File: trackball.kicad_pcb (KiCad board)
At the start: 4 copper layers, 65 x 85 mm, 255 parts, among them J2 ZX-PM2.0-2-4PY, Q1 XR2302, Q2 XR2302, Q4 XR2302, SW1 HX TC-5608-Y, SW2 HX TC-5608-Y, SW3 HX TC-5608-Y, SW4 HX TC-5608-Y, SW5 HX TC-5608-Y, SW6 HX TC-5608-Y, SW7 HX TC-5608-Y, SW8 HX TC-5608-Y, SW9 TS-1010-C-A, U1 USB-TYPE-C-017, U10 WS2812B, U11 WS2812B, U12 WS2812B, U13 WS2812B, U14 WS2812B, U15 WS2812B, U16 WS2812B, U17 WS2812B, U18 WS2812B, U19 WS2812B, U2 SY80004DQD, U20 WS2812B, U21 WS2812B, U3 SY80004DQD, U4 PMW3610, U5 PMW3610, U6 WS2812B, U7 WS2812B, U8 WS2812B, U9 WS2812B, X1 XL7EL89CKI-111YLC-32M

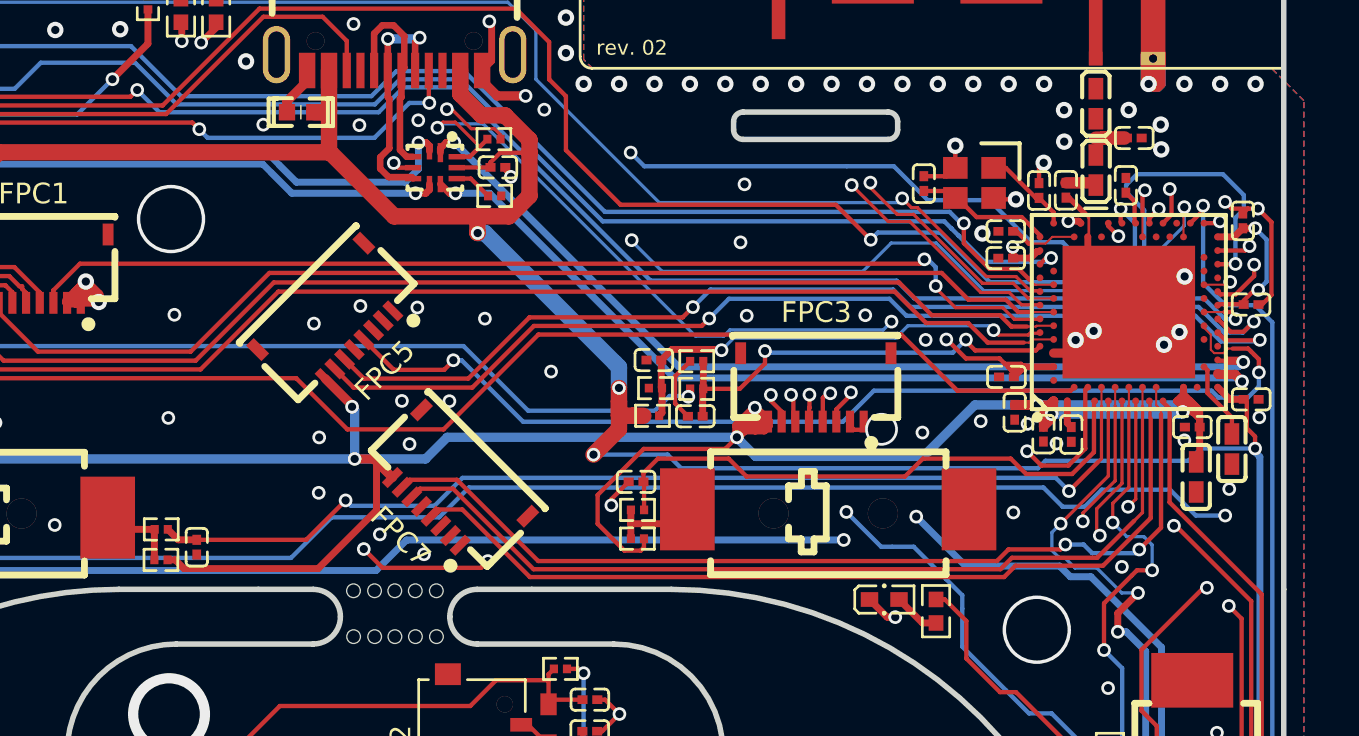
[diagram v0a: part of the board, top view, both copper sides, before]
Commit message: chore: refactoring
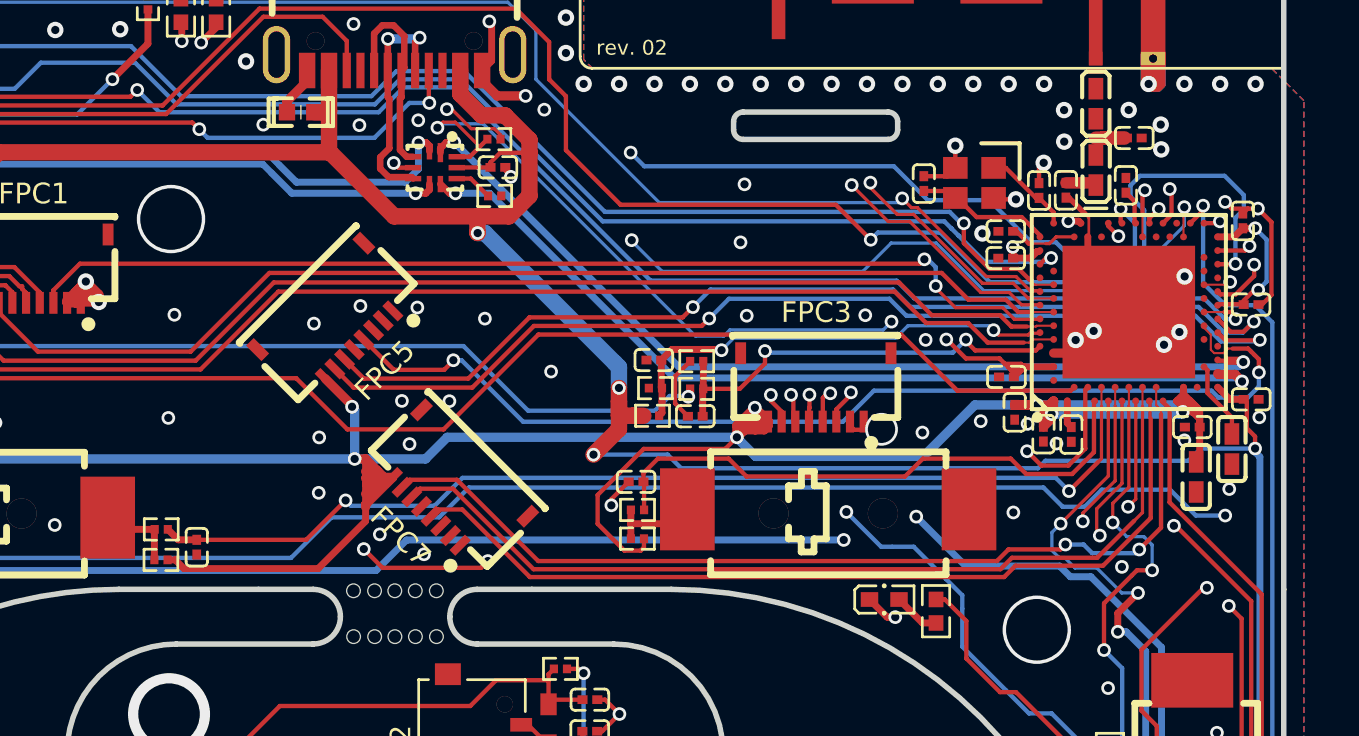
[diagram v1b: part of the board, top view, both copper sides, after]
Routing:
- net 1V8: track 321.0 -> 324.7 mm
